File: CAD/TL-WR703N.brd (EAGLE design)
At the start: 47.4 x 50 mm, 241 parts, among them T1 H1601CG, U1 AR9331-AL1A, U2 A3S56F40FTP

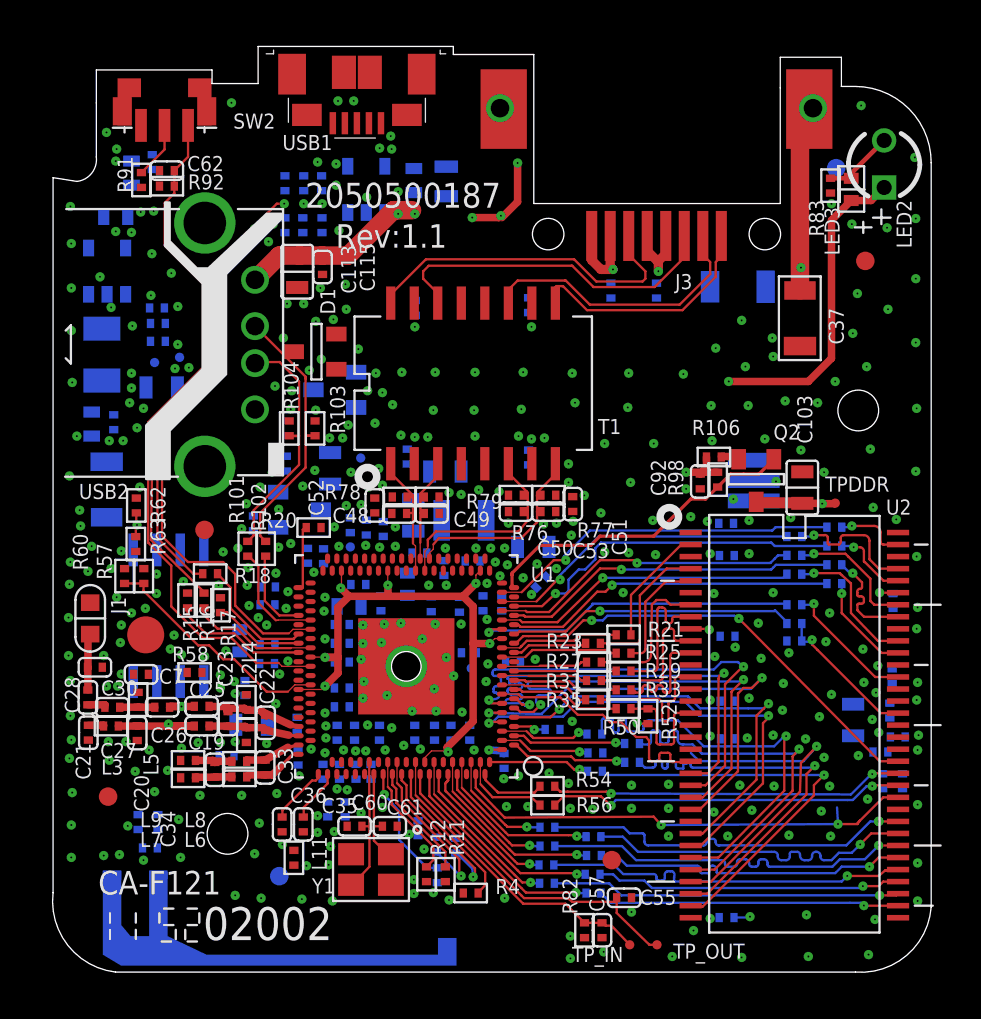
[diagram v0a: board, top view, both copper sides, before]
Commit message: Definitely good progress on top side!
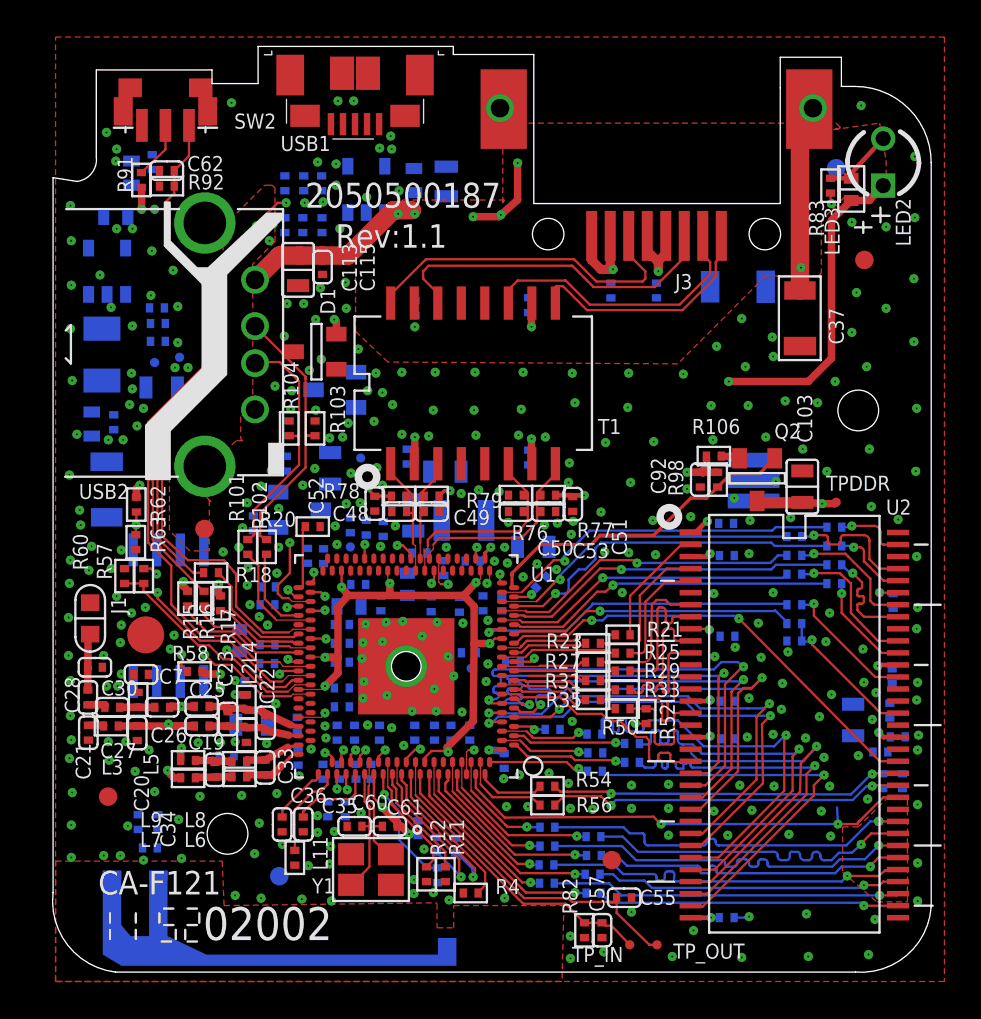
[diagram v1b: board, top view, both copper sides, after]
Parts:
- moved LED2 0.11 mm to (45.7, 44.2)
- moved R102 0.11 mm to (12.4, 23.5)
- moved C113 0.11 mm to (14.1, 38.4)
- moved USB1 0.11 mm to (17.2, 48.9)
- moved C48 0.10 mm to (19.6, 25.4)
- moved C49 0.10 mm to (21.3, 25.4)
- moved R101 0.10 mm to (11.4, 23.5)
- moved R17 0.10 mm to (9.91, 20.4)
- moved R52 0.10 mm to (32.9, 14.3)
- moved R63 0.10 mm to (5.33, 23.7)
- moved C52 0.10 mm to (18.2, 25.8)
- moved C92 0.10 mm to (35.8, 27.1)
- moved R15 0.10 mm to (8.13, 20.7)
- moved R16 0.10 mm to (9.02, 20.7)
- moved R20 0.07 mm to (14.9, 24.6)
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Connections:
- net S$452 renamed S$159
- removed net S$321: LED2.A, LED3.A
- removed net S$357: C35.2, U1.A69
- removed net S$367: J3.3, T1.16
- removed net S$370: C49.1, R79.1, T1.3, U1.A32
- removed net S$374: C50.2, R76.2, T1.6, U1.B27
- removed net S$379: Q2.1, R98.1, U1.A20
- removed net S$426: R49.1, U1.B18
- removed net S$49: C61.1, U1.A74, Y1.1
- removed net S$96: R17.2, U1.A53
- removed net VREF: U2.49
- new net $28: R79.2
- new net S$112: U1.A71
- new net S$114: C35.2, U1.A72
- new net S$115: L11.2, U1.A69
- new net S$116: U1.B59
- new net S$117: U1.B60
- new net S$118: U1.B61
- new net S$119: C61.1, U1.B63, Y1.1
- new net S$120: U1.B26
- new net S$121: U1.A19
- new net S$122: U1.B19
- new net S$123: U1.A33
- new net S$130: L9.2
- new net S$132: U1.A38
- new net S$133: U1.B39
- new net S$134: U1.B40
- new net S$135: U1.A49
- new net S$136: U1.A55
- new net S$137: R58.2
- new net S$138: U1.A56
- new net S$139: L4.2
- new net S$141: U1.A61
- new net S$145: U1.A25
- new net S$146: U1.A18
- new net S$147: R16.2, U1.B46
- new net S$148: R101.2, U1.B43
- new net S$150: R15.2, U1.A54
- new net S$151: T1.7
- new net S$152: U1.A48
- new net S$156: C22.2, C23.2, C25.2, L4.1, U1.A62
- new net S$161: D1.2
- new net S$162: J3.7, T1.11
- new net S$163: R83.1
- new net S$164: R91.1
- new net S$165: U1.B49
- new net S$17: L7.2
- new net S$18: U1.A70
- new net S$180: U1.B51
- new net S$186: U1.A57
- new net S$190: R62.1
- new net S$199: R57.1
- new net S$203: U1.B41
- new net S$228: R16.1
- new net S$252: J3.3, T1.16
- new net S$28: C49.1, R79.1, T1.3, U1.A32
- new net S$294: LED2.A, LED3.A
- new net S$331: T1.2
- new net S$409: U1.A30
- new net S$411: U1.A26
- new net S$416: R49.1, U1.B18
- new net S$417: U1.A58, U1.B13, U1.B21, U1.B31, U1.B36, U1.B47, U1.B69
- new net S$430: Q2.1, R98.1, U1.A20
- new net S$431: R29.2, U1.A11
- new net S$44: U2.49
- new net S$449: R17.2, U1.A53
- new net S$69: C51.2, R77.2
- new net S$71: C50.2, R76.2, T1.6, U1.B27
- new net S$84: R46.1, U1.B74
- new net S$86: C57.2, R82.2, TP_IN.1, U1.B68
- new net S$88: R12.2, U1.B65
- new net S$89: C60.2, U1.A73, Y1.3
- net GND: now also C61.2, U1.A74, U1.PAD
- net S$102: now also U1.B42; no longer R101.2, U1.B43
- net S$103: now also U1.B20; no longer U1.A58, U1.B13, U1.B21, U1.B31, U1.B36, U1.B47, U1.B69
- net S$109: now also R15.1; no longer R15.2, U1.A54
- net S$110: now also U1.B45; no longer R16.2, U1.B46
- net S$111: now also R17.1; no longer R16.1
- net S$15: now also U1.B67; no longer C57.2, R82.2, TP_IN.1, U1.B68
- net S$36: now also U1.A12; no longer R29.2, U1.A11
- net S$42: now also T1.10; no longer J3.7, T1.11
- net S$429: no longer U1.A18
- net S$48: now also U1.B62; no longer C60.2, U1.B63, Y1.3
- net S$51: now also U1.B64; no longer R12.2, U1.B65
- net S$67: now also U1.A84; no longer R46.1, U1.B74
- net S$78: now also R58.1; no longer C22.2, C23.2, C25.2, L4.1, U1.A62
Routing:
- net S$417: track 0.00 -> 32.7 mm, vias 1 -> 7
- net S$103: track 32.6 -> 0.76 mm, vias 7 -> 1
- net S$228: track 0.00 -> 23.3 mm
- net S$111: track 23.3 -> 0.67 mm
- net S$426: track 19.3 -> 0.00 mm, vias 1 -> 0
- net S$416: track 0.00 -> 19.3 mm
- net S$367: track 18.2 -> 0.00 mm
- net S$252: track 0.00 -> 18.2 mm, vias 1 -> 0
- net S$430: track 0.00 -> 17.6 mm, vias 1 -> 0
- net S$379: track 17.5 -> 0.00 mm
- net S$294: track 0.00 -> 17.1 mm
- net S$321: track 17.1 -> 0.00 mm, vias 1 -> 0
- net S$86: track 0.00 -> 16.8 mm, vias 1 -> 0
- net S$15: track 16.8 -> 1.16 mm, vias 0 -> 1
- net S$162: track 0.00 -> 15.3 mm
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- added copper zone on layer 1, net GND
- added copper zone on layer 1, net S$166
- added copper zone on layer 1, net S$167
- added copper zone on layer 1, net S$169
- added copper zone on layer 1, net S$170

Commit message: Looks like the top side is done!
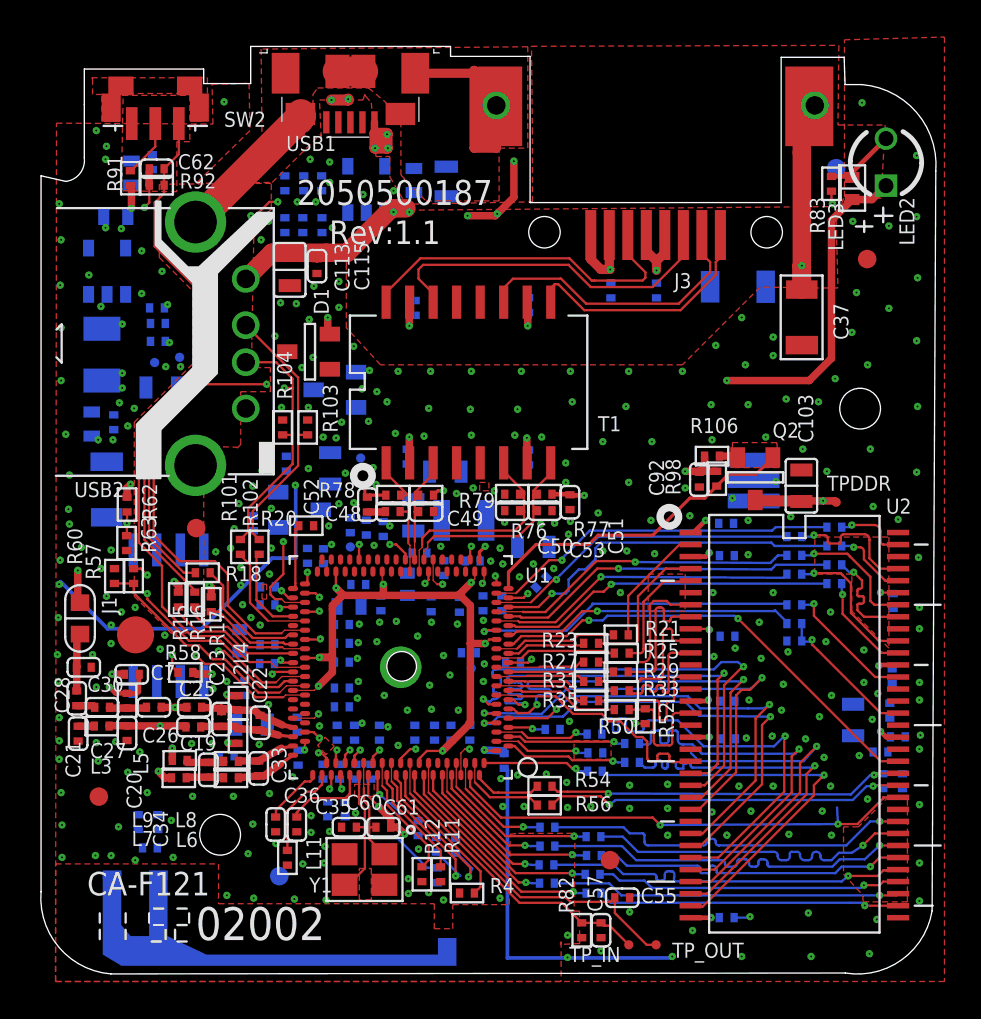
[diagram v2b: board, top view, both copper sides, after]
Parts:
- moved R91 0.61 mm to (5.04, 43.4)
- moved L5 0.60 mm to (4.86, 15.2)
- moved C28 0.60 mm to (2.14, 15.3)
- moved C30 0.60 mm to (2.52, 17.0)
- moved C62 0.56 mm to (6.46, 43.9)
- moved SW2 0.56 mm to (6.38, 46.3)
- moved R92 0.55 mm to (6.46, 43.0)
- moved C21 0.55 mm to (2.22, 13.4)
- moved C27 0.55 mm to (3.51, 14.8)
- moved C20 0.55 mm to (4.86, 13.4)
- moved GND 0.55 mm to (5.32, 18.7)
- moved J1 0.55 mm to (2.32, 19.6)
- moved R57 0.55 mm to (5.21, 21.9)
- moved R60 0.55 mm to (4.18, 21.9)
- moved R15 0.50 mm to (7.63, 20.6)
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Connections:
- removed net S$141: U1.A61
- removed net S$186: U1.A57
- removed net S$263: U1.B44
- removed net S$352: R39.2, U2.56
- removed net S$365: J3.6, T1.14
- new net S$124: R39.2
- new net S$125: U1.B55
- new net S$127: C34.2, L8.2, L9.1
- new net S$140: U1.A61
- new net S$157: T1.15
- new net S$171: U1.A77
- new net S$172: U2.56
- new net S$178: J1.2
- new net S$182: R101.1, R104.1, USB2.3
- new net S$238: U1.B44
- new net S$41: J3.6, T1.14
- new net S$93: C7.1
- new net S$96: U1.A57
- new net SHIELD: J3.S$1, USB1.S$1, USB1.S$2, USB1.S$3, USB1.S$4, USB1.S$5, USB1.S$6, USB2.S$1
- net GND: now also C103.2, C113.1, C115.1, C20.1, C21.1, C30.2, C36.1, C37.1, C49.2, C51.1, C55.2, C57.1, C62.1, C7.2, C92.1, D1.1, GND.1, L11.1, L5.2, R103.2, R104.2, R20.2, R4.2, R60.1, R92.1, USB1.GND, Y1.2, Y1.4
- net S$108: now also USB1.VBUS; no longer J3.S$1, USB1.S$1, USB1.S$2, USB1.S$3, USB1.S$4, USB1.S$5, USB1.S$6, USB2.S$1
- net S$70: now also L2.1; no longer C34.2, L8.2, L9.1
- net S$76: now also U1.B56; no longer R2.2, U1.A77
- net S$85: now also C48.1, C52.1; no longer R101.1, R104.1, USB2.3
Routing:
- net GND: track 6.00 -> 50.7 mm, vias 289 -> 308
- net S$263: track 30.6 -> 0.00 mm, vias 1 -> 0
- net S$238: track 0.00 -> 24.2 mm
- net SHIELD: track 0.00 -> 20.6 mm
- net S$41: track 0.00 -> 18.8 mm, vias 1 -> 0
- net S$365: track 18.6 -> 0.00 mm
- net S$182: track 0.00 -> 13.9 mm
- net S$85: track 13.6 -> 1.01 mm
- net S$171: track 0.00 -> 8.83 mm, vias 0 -> 1
- net S$76: track 8.69 -> 0.48 mm
- net S$352: track 5.62 -> 0.00 mm, vias 1 -> 0
- net S$108: track 0.00 -> 5.11 mm, vias 0 -> 3
- net S$96: track 0.00 -> 4.96 mm
- net S$172: track 0.00 -> 4.92 mm, vias 0 -> 1
- net S$186: track 4.80 -> 0.00 mm
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- added copper zone on layer 1, net S$107
- added copper zone on layer 1, net S$141
- added copper zone on layer 1, net S$173
- added copper zone on layer 1, net S$175
- added copper zone on layer 1, net S$176
- added copper zone on layer 1, net S$177
- added copper zone on layer 1, net S$179
- added copper zone on layer 1, net S$181
- added copper zone on layer 1, net S$183
- added copper zone on layer 1, net S$184
- added copper zone on layer 1, net S$186
- added copper zone on layer 1, net S$187
- added copper zone on layer 1, net SHIELD
- removed copper zone on layer 1, net S$170
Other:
- board size 47.4 x 50 mm -> 48.3 x 50.1 mm

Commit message: Completed layout reverse engineering!
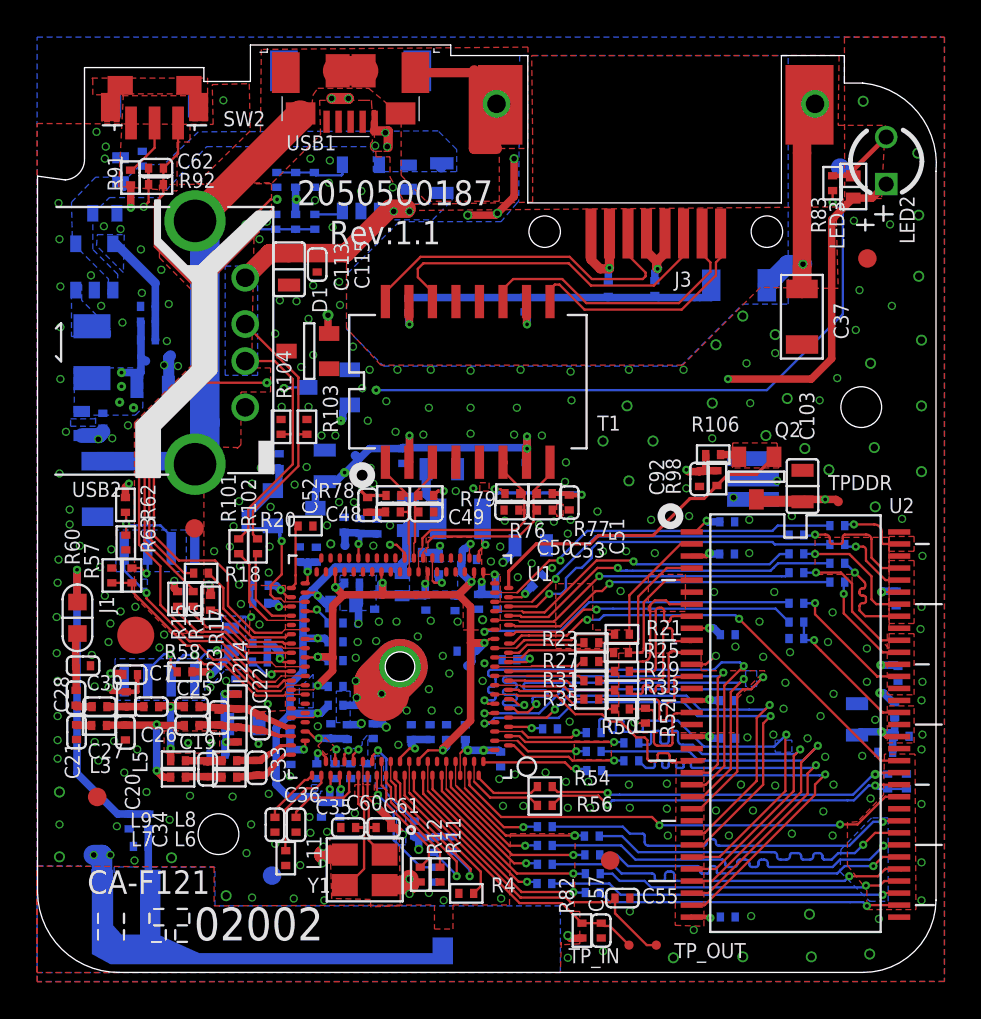
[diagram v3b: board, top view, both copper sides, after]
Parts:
- moved U5 0.73 mm to (3.09, 38.6)
- moved C107 0.62 mm to (4.51, 43.8)
- moved C112 0.62 mm to (3.66, 41.5)
- moved C111 0.59 mm to (3.55, 30.3)
- moved AN1 0.59 mm to (5.96, 5.78)
- moved C108 0.57 mm to (5.68, 44.4)
- moved L14 0.55 mm to (2.96, 34.0)
- moved C106 0.55 mm to (5.99, 34.6)
- moved R99 0.55 mm to (5.99, 35.6)
- moved C110 0.54 mm to (2.41, 30.1)
- moved R110 0.52 mm to (12.9, 41.0)
- moved C18 0.50 mm to (10.7, 15.9)
- moved C24 0.50 mm to (9.75, 12.3)
- moved R100 0.50 mm to (5.99, 36.5)
- moved TP3V3 0.50 mm to (5.86, 33.5)
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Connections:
- removed net S$109: R15.1
- removed net S$111: R17.1
- removed net S$124: R39.2
- removed net S$134: U1.B40
- removed net S$139: L4.2
- removed net S$140: U1.A61
- removed net S$146: U1.A18
- removed net S$151: T1.7
- removed net S$158: C25.1, C26.2
- removed net S$163: R83.1
- removed net S$168: C19.1, C20.2, L3.2
- removed net S$331: T1.2
- removed net S$411: U1.A26
- removed net S$417: U1.A58, U1.B13, U1.B21, U1.B31, U1.B36, U1.B47, U1.B69
- removed net S$48: U1.B62
- removed net S$69: C51.2, R77.2
- removed net S$70: L2.1
- new net S$126: C106.1, R100.2, R99.1, U5.5
- new net S$128: R109.2, R111.2, R112.2, U6.4
- new net S$142: R97.2
- new net S$143: R96.2
- new net S$154: R95.1
- new net S$192: C64.2, C66.2, U1.A84, U1.B1
- new net S$193: C45.2, R64.1, R65.2, R68.2, R71.1
- new net S$194: R107.2, U6.3
- new net S$216: C70.2, Q1.2, R93.2
- new net S$221: D2.2
- new net S$224: C46.1, C47.1, C84.2, Q1.3, T1.2, T1.7, TP2V0.1
- new net S$230: R83.1
- new net S$239: C106.2, C109.2, C110.1, C111.1, L14.1, R99.2, TP3V3.1
- new net S$265: R108.2, R109.1
- new net S$390: R59.1
- new net S$415: C4.2
- new net S$54: C51.2, R76.1, R77.2
- new net S$72: R82.1
- new net S$82: R14.2, R2.1, R3.1
- net GND: now also AN1.GND, C1.2, C100.1, C101.1, C102.1, C104.2, C105.2, C107.1, C108.1, C109.1, C11.1, C110.2, C111.2, C112.2, C114.2, C119.2, C12.1, C13.1, C14.1, C15.2, C16.1, C17.1, C18.2, C2.2, C24.2, C3.2, C31.2, C32.1, C35.1, C4.1, C46.2, C47.2, C5.2, C50.1, C53.2, C60.1, C63.1, C64.1, C65.2, C67.1, C70.1, C71.1, C73.2, C74.1, C75.2, C76.2, C77.1, C78.1, C79.2, C8.2, C80.2, C81.1, C82.1, C83.2, C84.1, C85.1, C86.1, C87.2, C88.2, C89.2, C9.1, C90.2, C91.1, C93.1, C94.1, C95.1, C96.1, C97.2, C98.2, C99.1, D2.1, E$9.GND$1, E$9.GND$2, E$9.GND$3, R100.1, R110.2, R111.1, R13.2, R15.1, R17.1, R53.1, R6.2, R7.2, TPGND.1, U3.4, U5.2, U6.2, USB2.4
- net S$102: now also C86.2
- net S$103: now also C5.1, C87.1, U1.B19
- net S$108: now also C107.2, C108.2, C112.1, C119.1, R113.1, U5.1, U5.4, U6.5
- net S$110: now also USB1.P$1, USB1.P$2; no longer U1.B45
- net S$112: now also L2.1; no longer U1.A71
- net S$116: now also R7.1
- net S$117: now also C88.1, C89.1, C90.1, R96.1, U1.B61, U1.B62
- net S$118: now also L14.2, U5.3; no longer U1.B61
- net S$120: now also C67.2, C71.2, C73.1, C74.2, C75.1, C76.1, C77.2, C78.2, C83.1, R94.2, TP1V2.1, U1.A26, U1.A58, U1.B13, U1.B21, U1.B31, U1.B36, U1.B47, U1.B69
- net S$121: now also C63.2
- net S$122: now also C81.2, U1.B45; no longer U1.B19
- net S$125: now also C91.2, R97.1
- net S$130: now also C25.1, C26.2
- net S$132: now also C101.2, C94.2, C95.2, TP2V5.1
- net S$133: now also C102.2, C96.2
- net S$135: now also C97.1
- net S$136: now also C98.1, R84.1
- net S$137: now also U3.7
- net S$138: now also R84.2
- net S$145: now also L13.2
- net S$15: now also C100.2, C99.2
- net S$152: now also C2.1
- net S$157: now also R64.2
- net S$159: now also U3.3
- net S$165: now also U3.1
- net S$17: now also C19.1, C20.2, L3.2
- net S$172: now also R39.2
- net S$178: now also C29.1, C31.1
- net S$18: now also C104.1, C105.1, C3.1, C38.1, C79.1, C80.1, C82.2, L1.2, L13.1, R94.1, U1.A61, U1.A71, U1.B40
- net S$180: now also U3.6
- net S$182: now also D2.3
- net S$199: now also U3.2
- net S$203: now also Q1.1, R93.1
- net S$228: now also R107.1, R108.1, R110.1
- net S$269: now also R113.2, U6.1
- net S$290: now also R65.1
- net S$291: now also R68.1
- net S$292: now also C45.1
- net S$36: now also C65.1
- net S$409: now also C93.2
- net S$42: now also R71.2
- net S$429: now also U1.A18
- net S$44: now also C16.2, C17.2, R59.2, R6.1
- net S$51: now also R14.1
- net S$53: now also C6.2, R55.2
- net S$60: now also C6.1, R55.1
- net S$67: now also C18.1, C24.1, C85.2, L4.2; no longer U1.A84
- net S$76: now also C1.1, L1.1
- net S$78: now also R95.2
- net S$83: now also AN1.RF, C29.2, C32.2; no longer C66.2, U1.B1
- net S$93: now also U3.8
- net S$96: now also U3.5
- net SHIELD: now also C114.1, USB2.S$2
- net VDD: now also C13.2, C14.2
- net VDDQ: now also C11.2, C12.2, C15.1, C8.1, C9.2
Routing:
- net S$120: track 0.72 -> 48.1 mm, vias 1 -> 11
- net S$18: track 0.79 -> 38.9 mm, vias 1 -> 4
- net S$230: track 0.00 -> 33.9 mm, vias 1 -> 2
- net S$417: track 32.3 -> 0.00 mm, vias 7 -> 0
- net SHIELD: track 20.6 -> 39.6 mm
- net S$224: track 0.00 -> 18.0 mm, vias 1 -> 4
- net S$193: track 0.00 -> 17.5 mm
- net S$178: track 1.76 -> 17.7 mm
- net GND: track 50.7 -> 35.8 mm, vias 308 -> 321
- net S$54: track 0.00 -> 7.29 mm, vias 1 -> 2
- net S$17: track 0.85 -> 7.73 mm, vias 1 -> 2
- net S$126: track 0.00 -> 6.26 mm, vias 1 -> 0
- net S$3: track 18.1 -> 23.0 mm
- net S$289: track 4.86 -> 0.00 mm, vias 3 -> 0
- net S$192: track 0.00 -> 4.73 mm, vias 0 -> 2
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- added copper zone on layer 16, net GND
- added copper zone on layer 1, net S$108
- added copper zone on layer 16, net S$108
- added copper zone on layer 16, net S$109
- added copper zone on layer 16, net S$111
- added copper zone on layer 16, net S$117
- added copper zone on layer 16, net S$118
- added copper zone on layer 16, net S$124
- added copper zone on layer 16, net S$129
- added copper zone on layer 16, net S$134
- added copper zone on layer 1, net S$139
- added copper zone on layer 1, net S$140
- added copper zone on layer 16, net S$146
- added copper zone on layer 1, net S$151
- added copper zone on layer 1, net S$153
- added copper zone on layer 16, net S$155
- added copper zone on layer 16, net S$158
- added copper zone on layer 16, net S$163
- added copper zone on layer 16, net S$168
- added copper zone on layer 1, net S$170
- added copper zone on layer 16, net S$174
- added copper zone on layer 16, net S$18
- added copper zone on layer 1, net S$185
- added copper zone on layer 1, net S$188
- added copper zone on layer 1, net S$191
- added copper zone on layer 16, net S$195
- added copper zone on layer 16, net S$196
- added copper zone on layer 16, net S$197
- added copper zone on layer 1, net S$198
- added copper zone on layer 1, net S$200
- added copper zone on layer 16, net S$201
- added copper zone on layer 16, net S$239
- added copper zone on layer 16, net S$269
- added copper zone on layer 16, net S$48
- added copper zone on layer 16, net S$69
- added copper zone on layer 16, net S$70
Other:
- board size 48.3 x 50.1 mm -> 48.5 x 50.1 mm
